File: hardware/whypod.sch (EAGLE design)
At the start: 13 parts, among them IC1 IC_USBLC6-2, X2 USB-A-S, Y1 CRYSTAL-GROUNDEDSMD-5X3.2

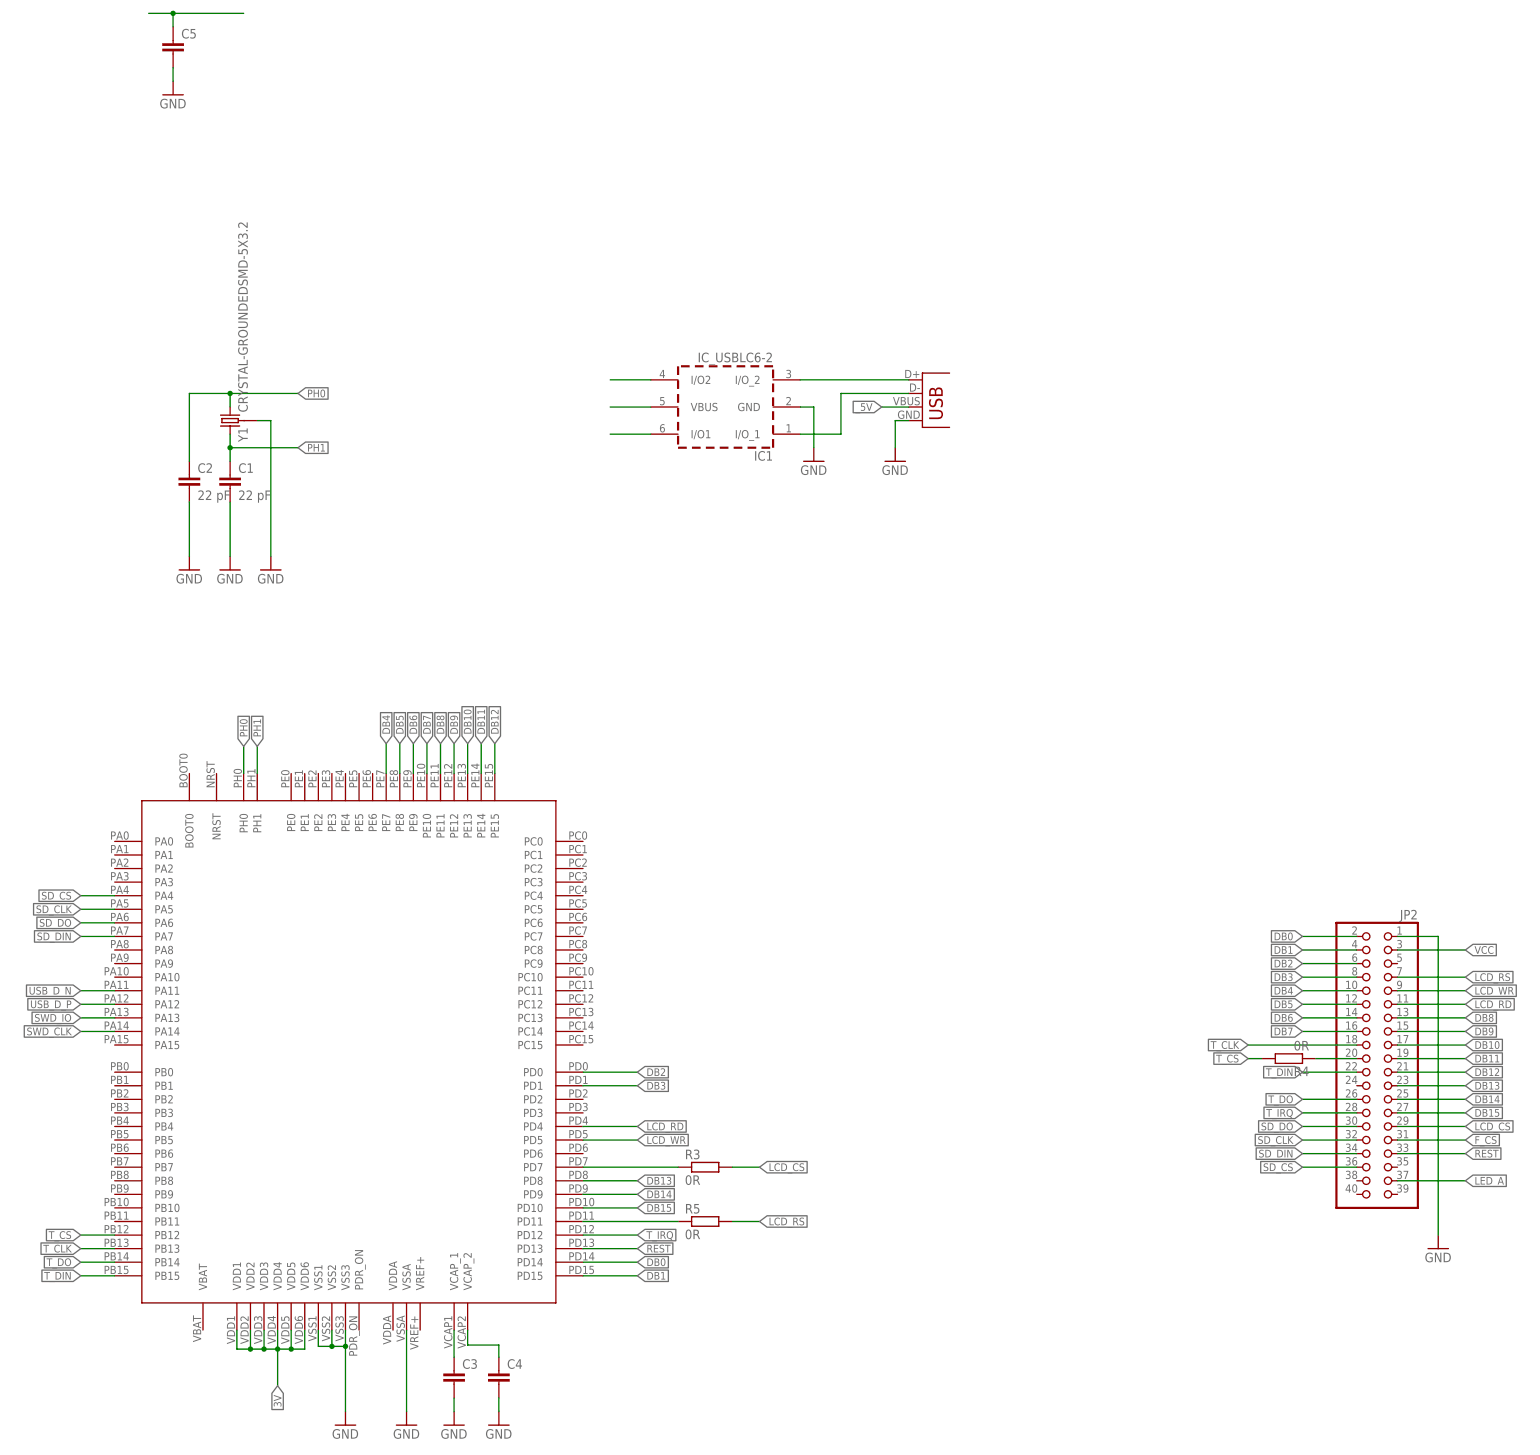
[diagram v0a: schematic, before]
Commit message: Hardware updates
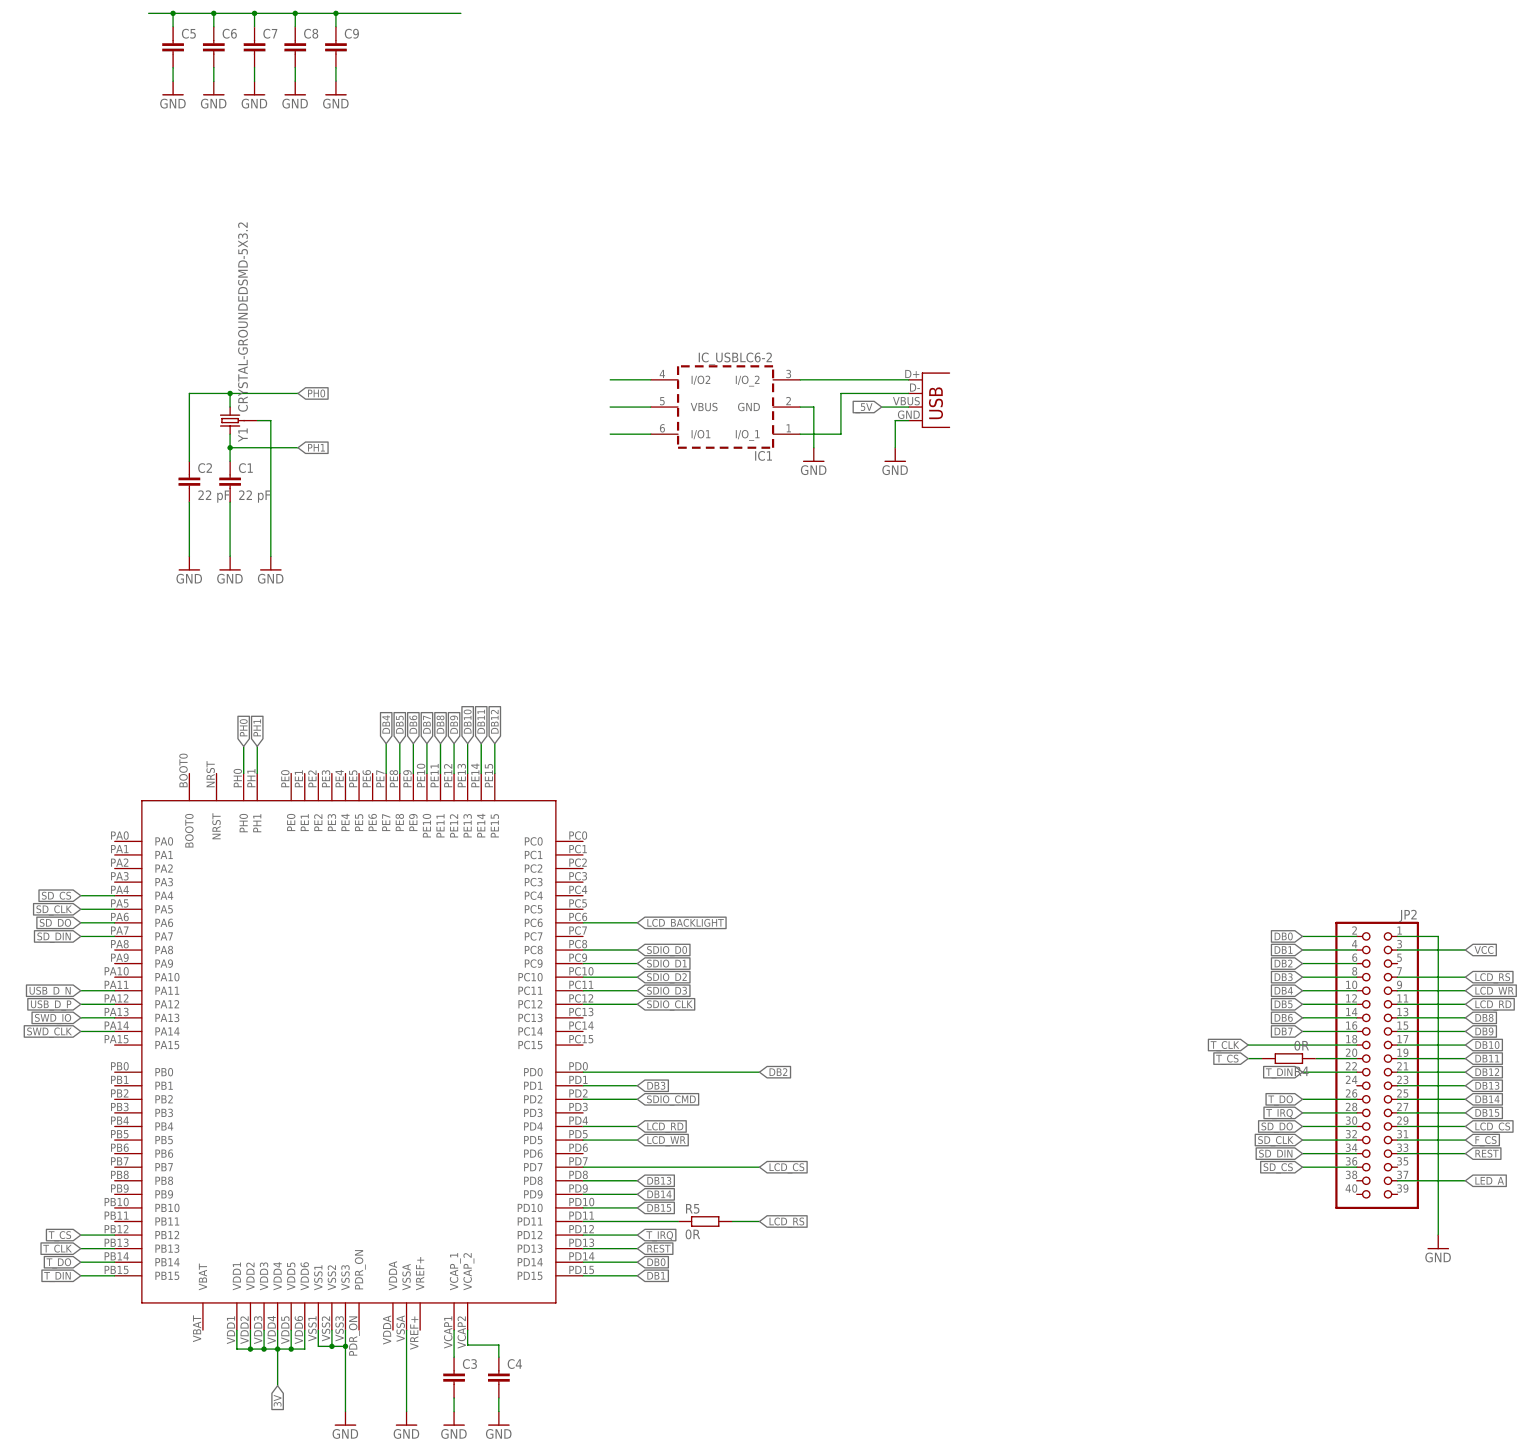
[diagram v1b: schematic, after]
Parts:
- removed R3: 0R, rcl:R-EU_R0603
- added C6, C7, C8, C9: (no value), rcl:C-EUC0603
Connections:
- removed net N$5: R3.1, U$2.PD7
- new net LCD_BACKLIGHT: U$2.PC6
- new net SDIO_CLK: U$2.PC12
- new net SDIO_CMD: U$2.PD2
- new net SDIO_D0: U$2.PC8
- new net SDIO_D1: U$2.PC9
- new net SDIO_D2: U$2.PC10
- new net SDIO_D3: U$2.PC11
- net 3V: now also C6.1, C7.1, C8.1, C9.1
- net GND: now also C6.2, C7.2, C8.2, C9.2
- net LCD_CS: now also U$2.PD7; no longer R3.2
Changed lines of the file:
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@@
 <part name="GND2" library="supply1" deviceset="GND" device=""/>
 <part name="GND3" library="supply1" deviceset="GND" device=""/>
-<part name="R3" library="rcl" deviceset="R-EU_" device="R0603" value="0R"/>
 <part name="C1" library="rcl" deviceset="C-EU" device="C0603" value="22 pF"/>
 <part name="C2" library="rcl" deviceset="C-EU" device="C0603" value="22 pF"/>
@@
 <part name="IC1" library="dp_devices" deviceset="IC_USBLC6-2" device=""/>
 <part name="GND10" library="supply1" deviceset="GND" device=""/>
+<part name="C6" library="rcl" deviceset="C-EU" device="C0603"/>
+<part name="GND11" library="supply1" deviceset="GND" device=""/>
+<part name="C7" library="rcl" deviceset="C-EU" device="C0603"/>
+<part name="GND12" library="supply1" deviceset="GND" device=""/>
+<part name="C8" library="rcl" deviceset="C-EU" device="C0603"/>
+<part name="GND13" library="supply1" deviceset="GND" device=""/>
+<part name="C9" library="rcl" deviceset="C-EU" device="C0603"/>
+<part name="GND14" library="supply1" deviceset="GND" device=""/>
 </parts>
 <sheets>
@@
 <instance part="GND2" gate="1" x="201.93" y="-45.72"/>
 <instance part="GND3" gate="1" x="213.36" y="-45.72"/>
-<instance part="R3" gate="G$1" x="269.24" y="2.54"/>
 <instance part="C1" gate="G$1" x="180.34" y="132.08"/>
 <instance part="C2" gate="G$1" x="172.72" y="132.08"/>
@@
 <instance part="IC1" gate="G$1" x="264.16" y="152.4" rot="R180"/>
 <instance part="GND10" gate="1" x="289.56" y="134.62"/>
+<instance part="C6" gate="G$1" x="177.292" y="213.36"/>
+<instance part="GND11" gate="1" x="177.292" y="203.2"/>
+<instance part="C7" gate="G$1" x="184.912" y="213.36"/>
+<instance part="GND12" gate="1" x="184.912" y="203.2"/>
+<instance part="C8" gate="G$1" x="192.532" y="213.36"/>
+<instance part="GND13" gate="1" x="192.532" y="203.2"/>
+<instance part="C9" gate="G$1" x="200.152" y="213.36"/>
+<instance part="GND14" gate="1" x="200.152" y="203.2"/>
 </instances>
 <busses>
@@
 <wire x1="289.56" y1="144.78" x2="289.56" y2="137.16" width="0.1524" layer="91"/>
 </segment>
+<segment>
+<pinref part="C6" gate="G$1" pin="2"/>
+<pinref part="GND11" gate="1" pin="GND"/>
+<wire x1="177.292" y1="205.74" x2="177.292" y2="208.28" width="0.1524" layer="91"/>
+</segment>
+<segment>
+<pinref part="C7" gate="G$1" pin="2"/>
+<pinref part="GND12" gate="1" pin="GND"/>
+<wire x1="184.912" y1="205.74" x2="184.912" y2="208.28" width="0.1524" layer="91"/>
+</segment>
+<segment>
+<pinref part="C8" gate="G$1" pin="2"/>
+<pinref part="GND13" gate="1" pin="GND"/>
+<wire x1="192.532" y1="205.74" x2="192.532" y2="208.28" width="0.1524" layer="91"/>
+</segment>
+<segment>
+<pinref part="C9" gate="G$1" pin="2"/>
+<pinref part="GND14" gate="1" pin="GND"/>
+<wire x1="200.152" y1="205.74" x2="200.152" y2="208.28" width="0.1524" layer="91"/>
+</segment>
 </net>
 <net name="DB0" class="0">
@@
 </segment>
 <segment>
+<label x="279.4" y="20.32" size="1.4224" layer="95" xref="yes"/>
 <pinref part="U$2" gate="G$1" pin="PD0"/>
-<wire x1="246.38" y1="20.32" x2="256.54" y2="20.32" width="0.1524" layer="91"/>
-<label x="256.54" y="20.32" size="1.4224" layer="95" xref="yes"/>
+<wire x1="279.4" y1="20.32" x2="246.38" y2="20.32" width="0.1524" layer="91"/>
 </segment>
 </net>
@@
 </segment>
 <segment>
-<pinref part="R3" gate="G$1" pin="2"/>
-<wire x1="274.32" y1="2.54" x2="279.4" y2="2.54" width="0.1524" layer="91"/>
 <label x="279.4" y="2.54" size="1.4224" layer="95" xref="yes"/>
+<pinref part="U$2" gate="G$1" pin="PD7"/>
+<wire x1="246.38" y1="2.54" x2="279.4" y2="2.54" width="0.1524" layer="91"/>
 </segment>
 </net>
@@
 <wire x1="246.38" y1="-10.16" x2="256.54" y2="-10.16" width="0.1524" layer="91"/>
 <label x="256.54" y="-10.16" size="1.4224" layer="95" xref="yes"/>
-</segment>
-</net>
-<net name="N$5" class="0">
-<segment>
-<pinref part="U$2" gate="G$1" pin="PD7"/>
-<pinref part="R3" gate="G$1" pin="1"/>
-<wire x1="264.16" y1="2.54" x2="246.38" y2="2.54" width="0.1524" layer="91"/>
 </segment>
 </net>
@@
 <wire x1="165.1" y1="218.44" x2="169.672" y2="218.44" width="0.1524" layer="91"/>
 <pinref part="C5" gate="G$1" pin="1"/>
-<wire x1="169.672" y1="218.44" x2="182.88" y2="218.44" width="0.1524" layer="91"/>
+<wire x1="169.672" y1="218.44" x2="177.292" y2="218.44" width="0.1524" layer="91"/>
+<wire x1="177.292" y1="218.44" x2="184.912" y2="218.44" width="0.1524" layer="91"/>
+<wire x1="184.912" y1="218.44" x2="192.532" y2="218.44" width="0.1524" layer="91"/>
+<wire x1="192.532" y1="218.44" x2="200.152" y2="218.44" width="0.1524" layer="91"/>
+<wire x1="200.152" y1="218.44" x2="223.52" y2="218.44" width="0.1524" layer="91"/>
 <wire x1="169.672" y1="215.9" x2="169.672" y2="218.44" width="0.1524" layer="91"/>
 <junction x="169.672" y="218.44"/>
+<pinref part="C6" gate="G$1" pin="1"/>
+<wire x1="177.292" y1="215.9" x2="177.292" y2="218.44" width="0.1524" layer="91"/>
+<junction x="177.292" y="218.44"/>
+<pinref part="C7" gate="G$1" pin="1"/>
+<wire x1="184.912" y1="215.9" x2="184.912" y2="218.44" width="0.1524" layer="91"/>
+<junction x="184.912" y="218.44"/>
+<pinref part="C8" gate="G$1" pin="1"/>
+<wire x1="192.532" y1="215.9" x2="192.532" y2="218.44" width="0.1524" layer="91"/>
+<junction x="192.532" y="218.44"/>
+<pinref part="C9" gate="G$1" pin="1"/>
+<wire x1="200.152" y1="215.9" x2="200.152" y2="218.44" width="0.1524" layer="91"/>
+<junction x="200.152" y="218.44"/>
 </segment>
 </net>
@@
 </segment>
 </net>
+<net name="LCD_BACKLIGHT" class="0">
+<segment>
+<pinref part="U$2" gate="G$1" pin="PC6"/>
+<wire x1="246.38" y1="48.26" x2="256.54" y2="48.26" width="0.1524" layer="91"/>
+<label x="256.54" y="48.26" size="1.4224" layer="95" xref="yes"/>
+</segment>
+</net>
+<net name="SDIO_D0" class="0">
+<segment>
+<pinref part="U$2" gate="G$1" pin="PC8"/>
+<wire x1="246.38" y1="43.18" x2="256.54" y2="43.18" width="0.1524" layer="91"/>
+<label x="256.54" y="43.18" size="1.4224" layer="95" xref="yes"/>
+</segment>
+</net>
+<net name="SDIO_D1" class="0">
+<segment>
+<pinref part="U$2" gate="G$1" pin="PC9"/>
+<wire x1="246.38" y1="40.64" x2="256.54" y2="40.64" width="0.1524" layer="91"/>
+<label x="256.54" y="40.64" size="1.4224" layer="95" xref="yes"/>
+</segment>
+</net>
+<net name="SDIO_D2" class="0">
+<segment>
+<pinref part="U$2" gate="G$1" pin="PC10"/>
+<wire x1="246.38" y1="38.1" x2="256.54" y2="38.1" width="0.1524" layer="91"/>
+<label x="256.54" y="38.1" size="1.4224" layer="95" xref="yes"/>
+</segment>
+</net>
+<net name="SDIO_D3" class="0">
+<segment>
+<pinref part="U$2" gate="G$1" pin="PC11"/>
+<wire x1="246.38" y1="35.56" x2="256.54" y2="35.56" width="0.1524" layer="91"/>
+<label x="256.54" y="35.56" size="1.4224" layer="95" xref="yes"/>
+</segment>
+</net>
+<net name="SDIO_CLK" class="0">
+<segment>
+<pinref part="U$2" gate="G$1" pin="PC12"/>
+<wire x1="246.38" y1="33.02" x2="256.54" y2="33.02" width="0.1524" layer="91"/>
+<label x="256.54" y="33.02" size="1.4224" layer="95" xref="yes"/>
+</segment>
+</net>
+<net name="SDIO_CMD" class="0">
+<segment>
+<pinref part="U$2" gate="G$1" pin="PD2"/>
+<wire x1="246.38" y1="15.24" x2="256.54" y2="15.24" width="0.1524" layer="91"/>
+<label x="256.54" y="15.24" size="1.4224" layer="95" xref="yes"/>
+</segment>
+</net>
